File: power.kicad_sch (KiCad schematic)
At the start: 45 parts, among them U4 MIC5504-3.3YM5-TR

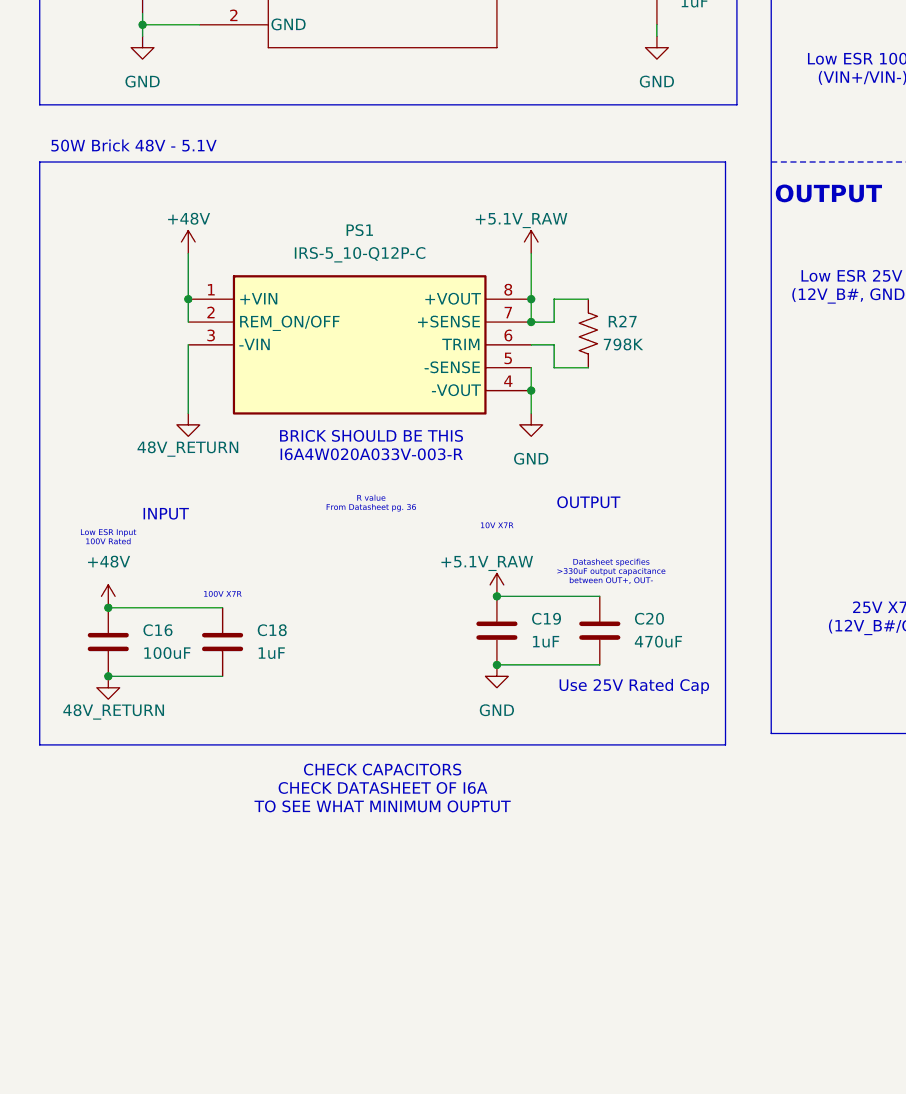
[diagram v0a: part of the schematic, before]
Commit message: updated some of nicks requested changes
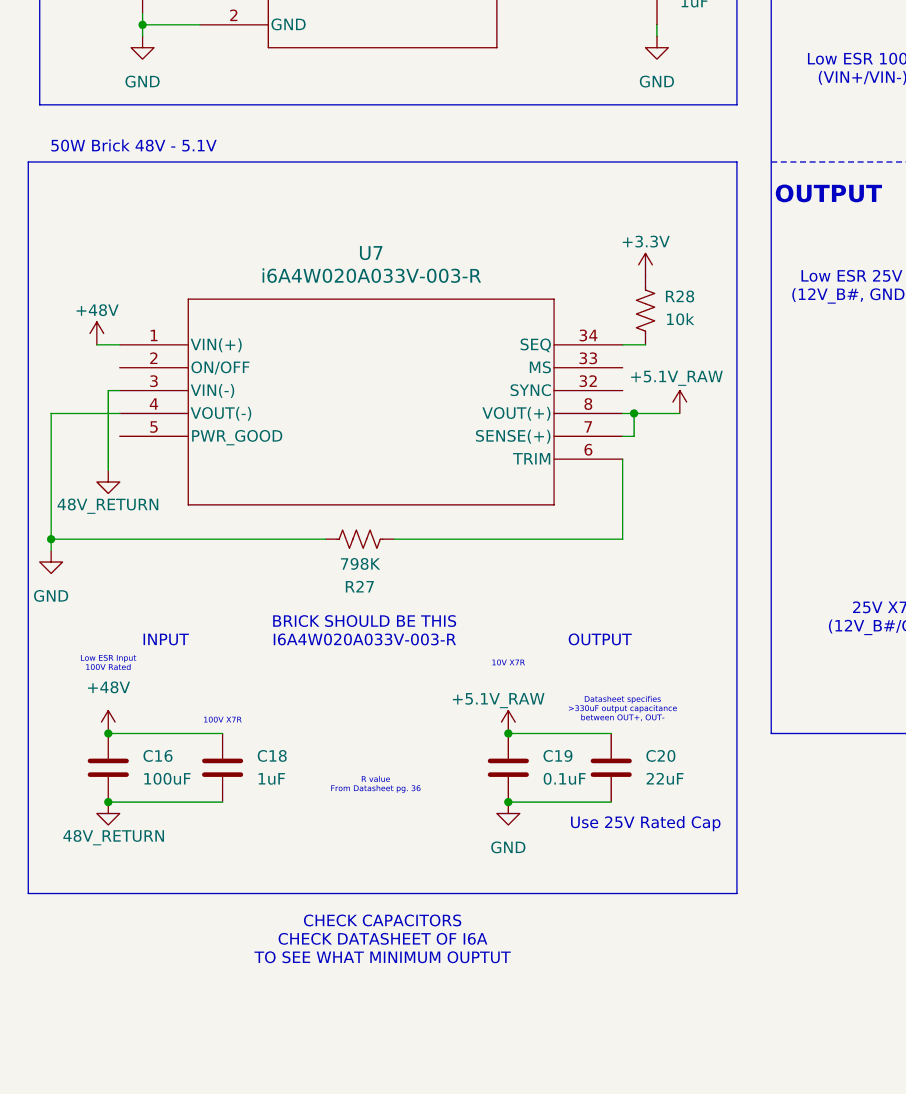
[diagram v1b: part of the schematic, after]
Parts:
- removed PS1: IRS-5_10-Q12P-C, IRS510Q12PC, symbol IRS-5_10-Q12P-C:IRS-5_10-Q12P-C
- added R28: 10k, symbol Device:R_US
- added U7: i6A4W020A033V-003-R, i6A4W_DIP_FULL_TDK, symbol 2026-10-14_21-27-49:i6A4W020A033V-003-R
- B2, B3, B4, B5: footprint E48SC12030NRFH -> rov_power:E48SC12030NRFH
- C17, C21, U4: footprint SOT-23-5_MC_MCH -> rov_power:SOT-23-5_MC_MCH
- C19: value 1uF -> 0.1uF
- C20: value 470uF -> 22uF
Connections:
- net +3.3V: now also R28.1
- net +48V: now also U7.1 (VIN(+))
- net +5.1V_RAW: now also U7.7 (SENSE(+)), U7.8 (VOUT(+)); no longer R27.2
- net 48V_RETURN: now also U7.3 (VIN(-))
- net GND: now also R27.2, U7.4 (VOUT(-))
- net at R27.1: now also U7.6 (TRIM)
- new net: R28.2, U7.34 (SEQ)
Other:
- moved on the sheet: C16, C18, C19, C20, R27
